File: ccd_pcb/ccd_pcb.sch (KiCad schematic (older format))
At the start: 19 parts

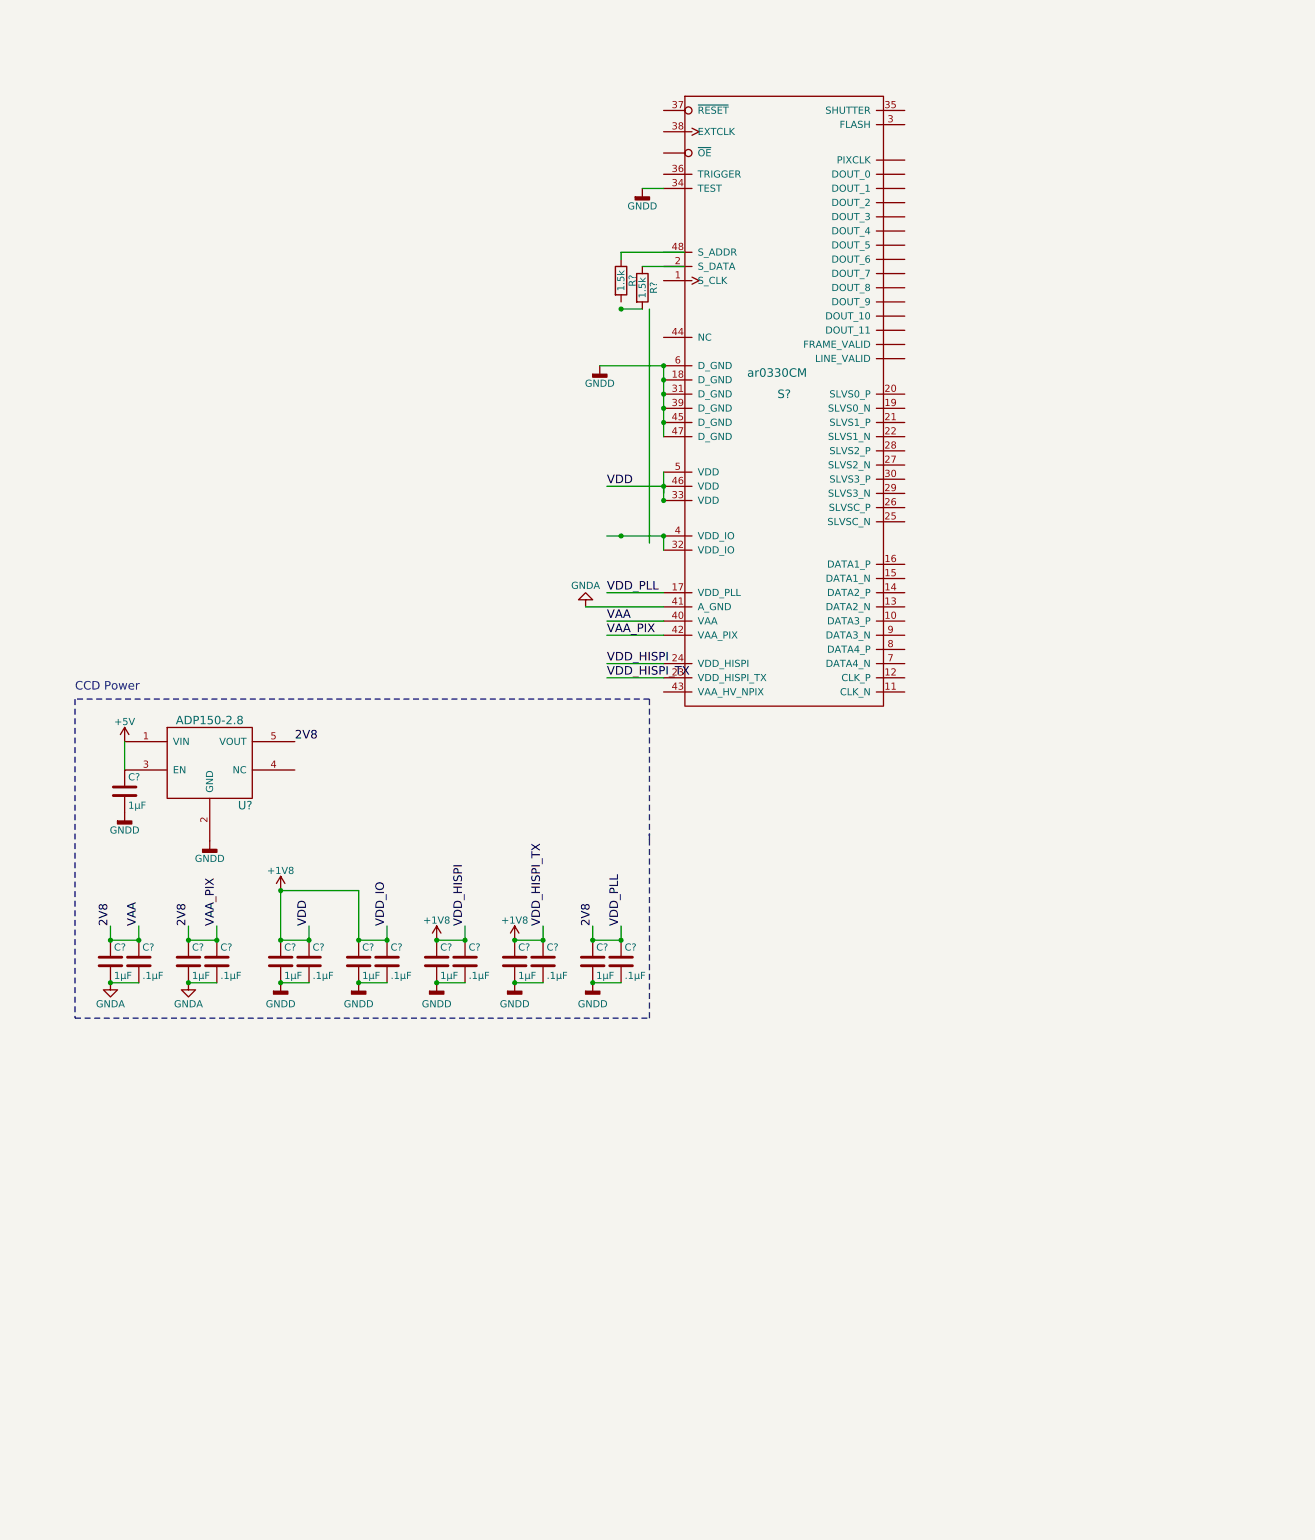
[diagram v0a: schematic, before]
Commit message: do more scematics work
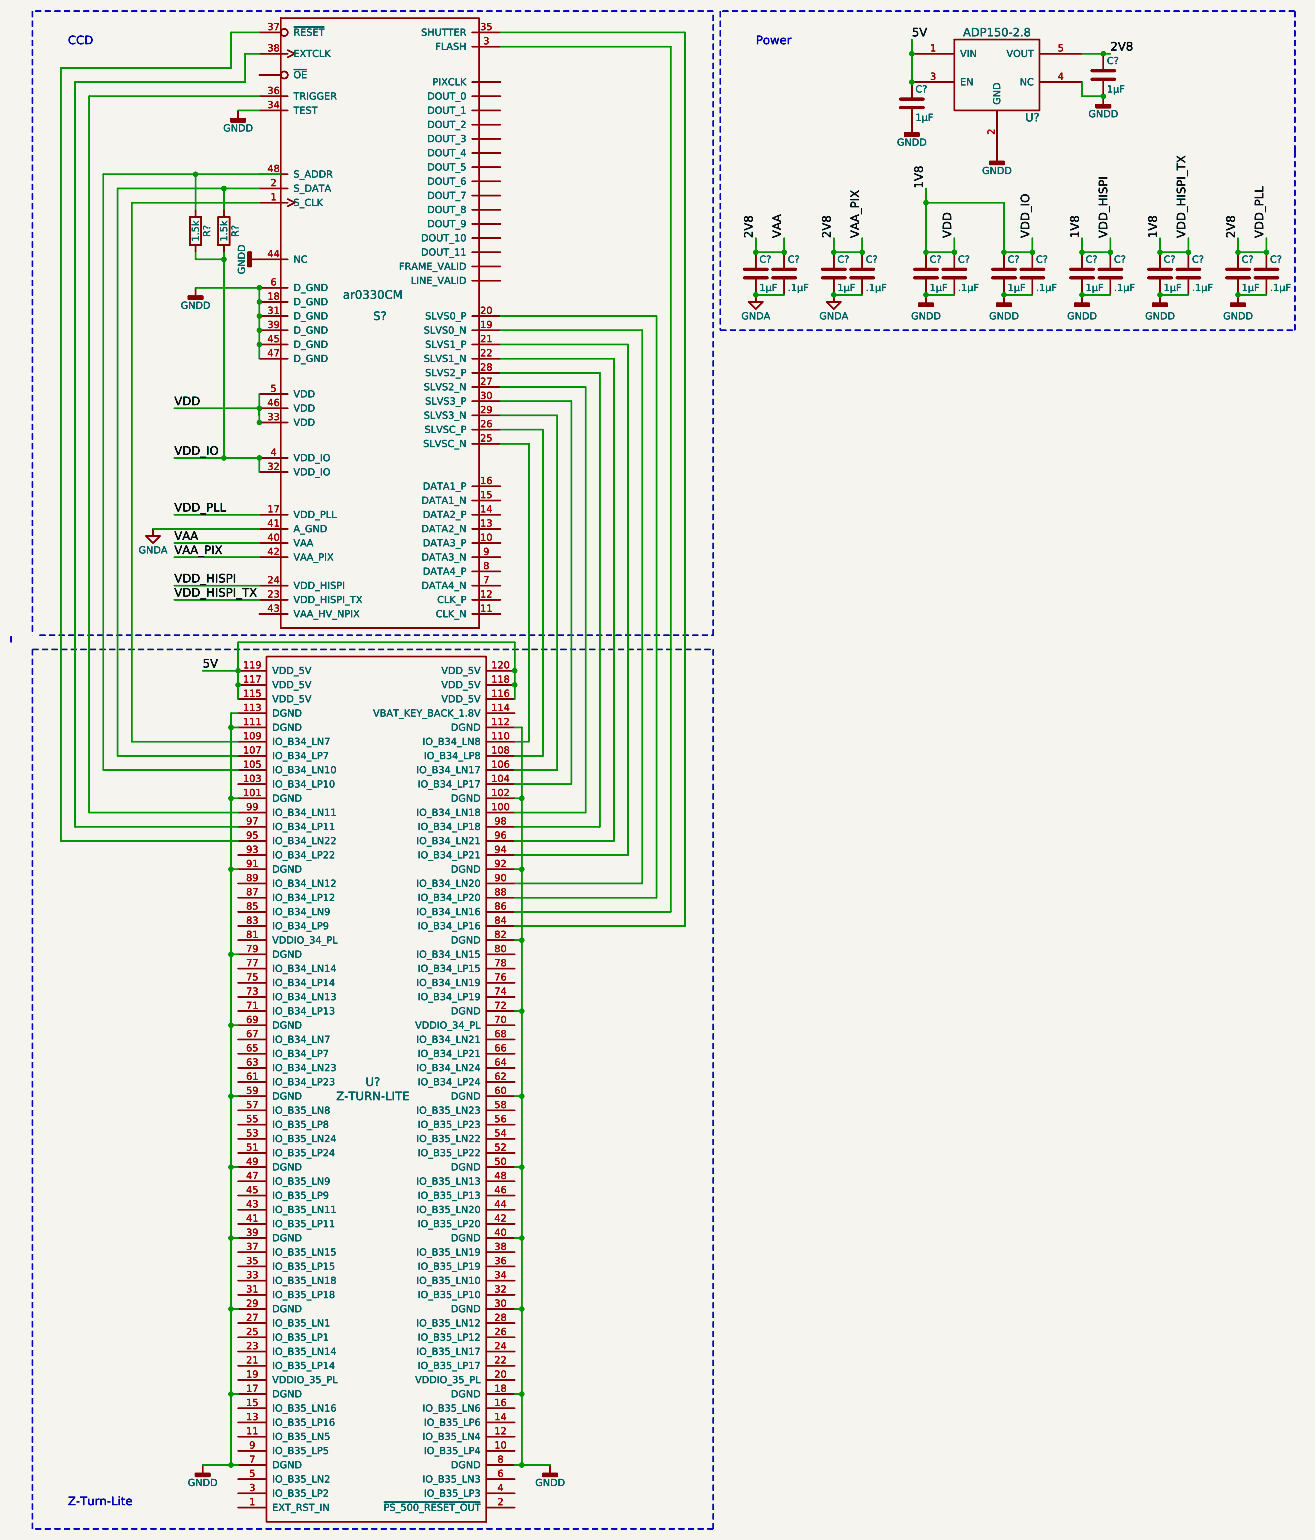
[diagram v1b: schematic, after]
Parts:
- added C? (x10): 1µF, symbol C
- added C? (x7): .1µF, symbol C
- added R? (x2): 1.5k, symbol R
- added S?: ar0330CM, symbol ar0330CM
- added U? (x2): Z-TURN-LITE, symbol Z-TURN-LITE
- added U?: ADP150-2.8, symbol ADP150-2.8
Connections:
- net labels added: 1V8, 5V
- net labels removed: +1V8, +5V
- wire segments 47 -> 278
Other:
- note added: "CCD\n"
- note added: "Power\n"
- note added: "Z-Turn-Lite\n"
- note removed: "CCD Power\n"
- moved on the sheet: C?, R?, S?, U?

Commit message: route power for plugin connector
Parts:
- added C?: PCIe-36-Axiom, symbol PCIe-36-Axiom
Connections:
- wire segments 278 -> 158
